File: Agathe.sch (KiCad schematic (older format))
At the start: 153 parts, among them SW1 SW_Push, U1 ATmega32U4-AU, U2 PRTR5V0U2X, Y1 Crystal_GND24_Small

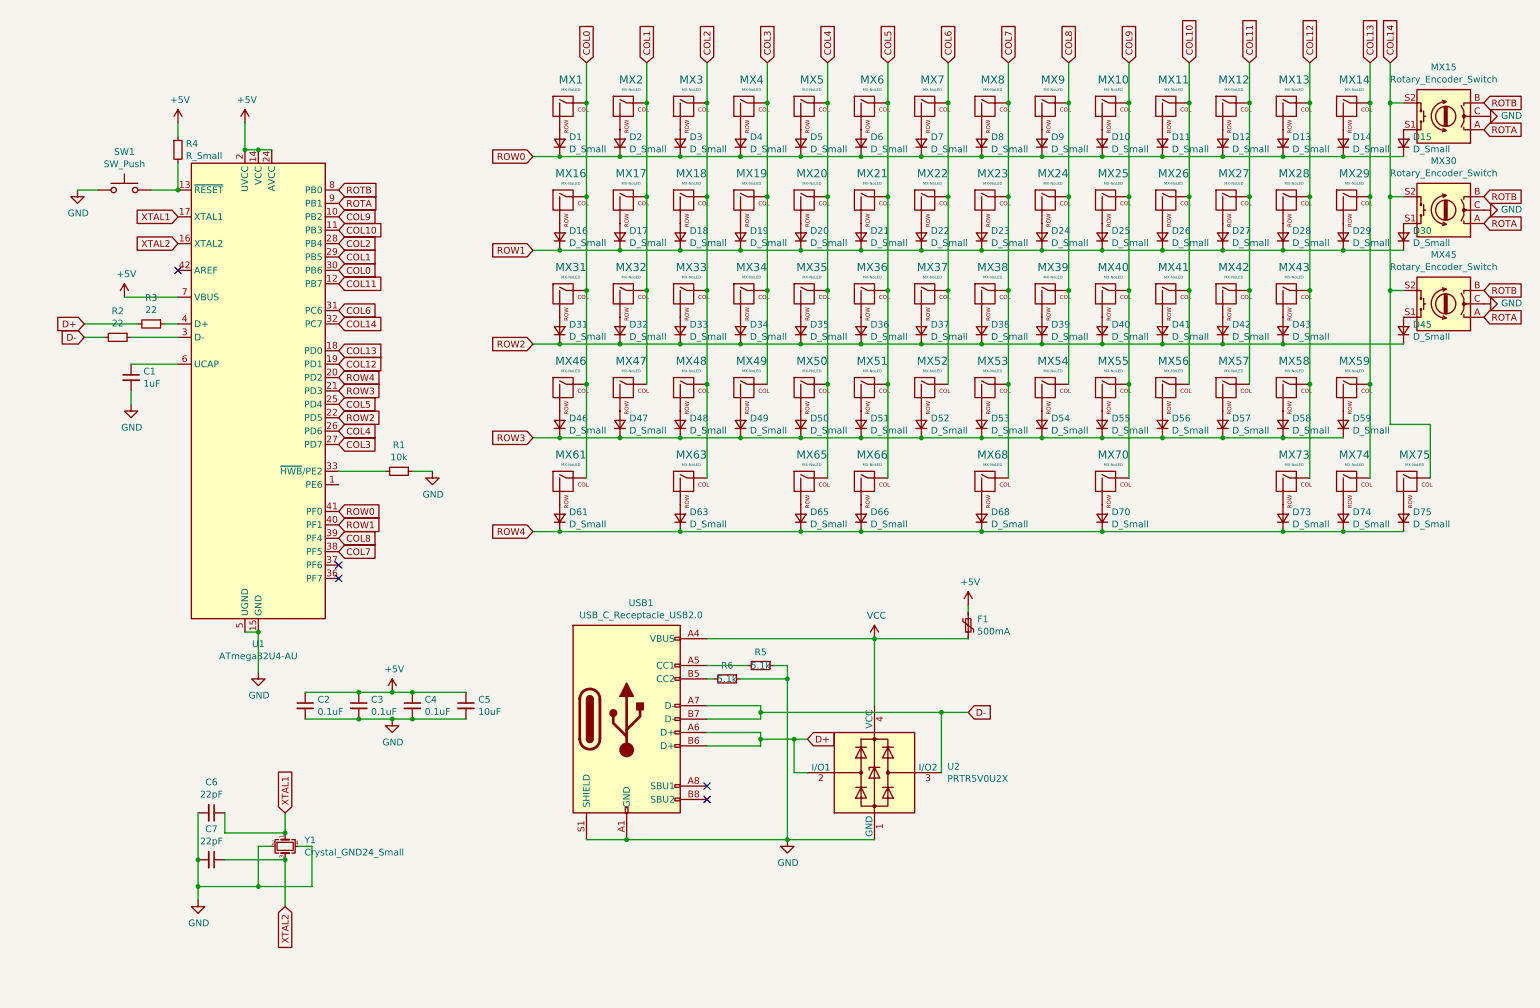
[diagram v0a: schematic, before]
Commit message: Add underglow
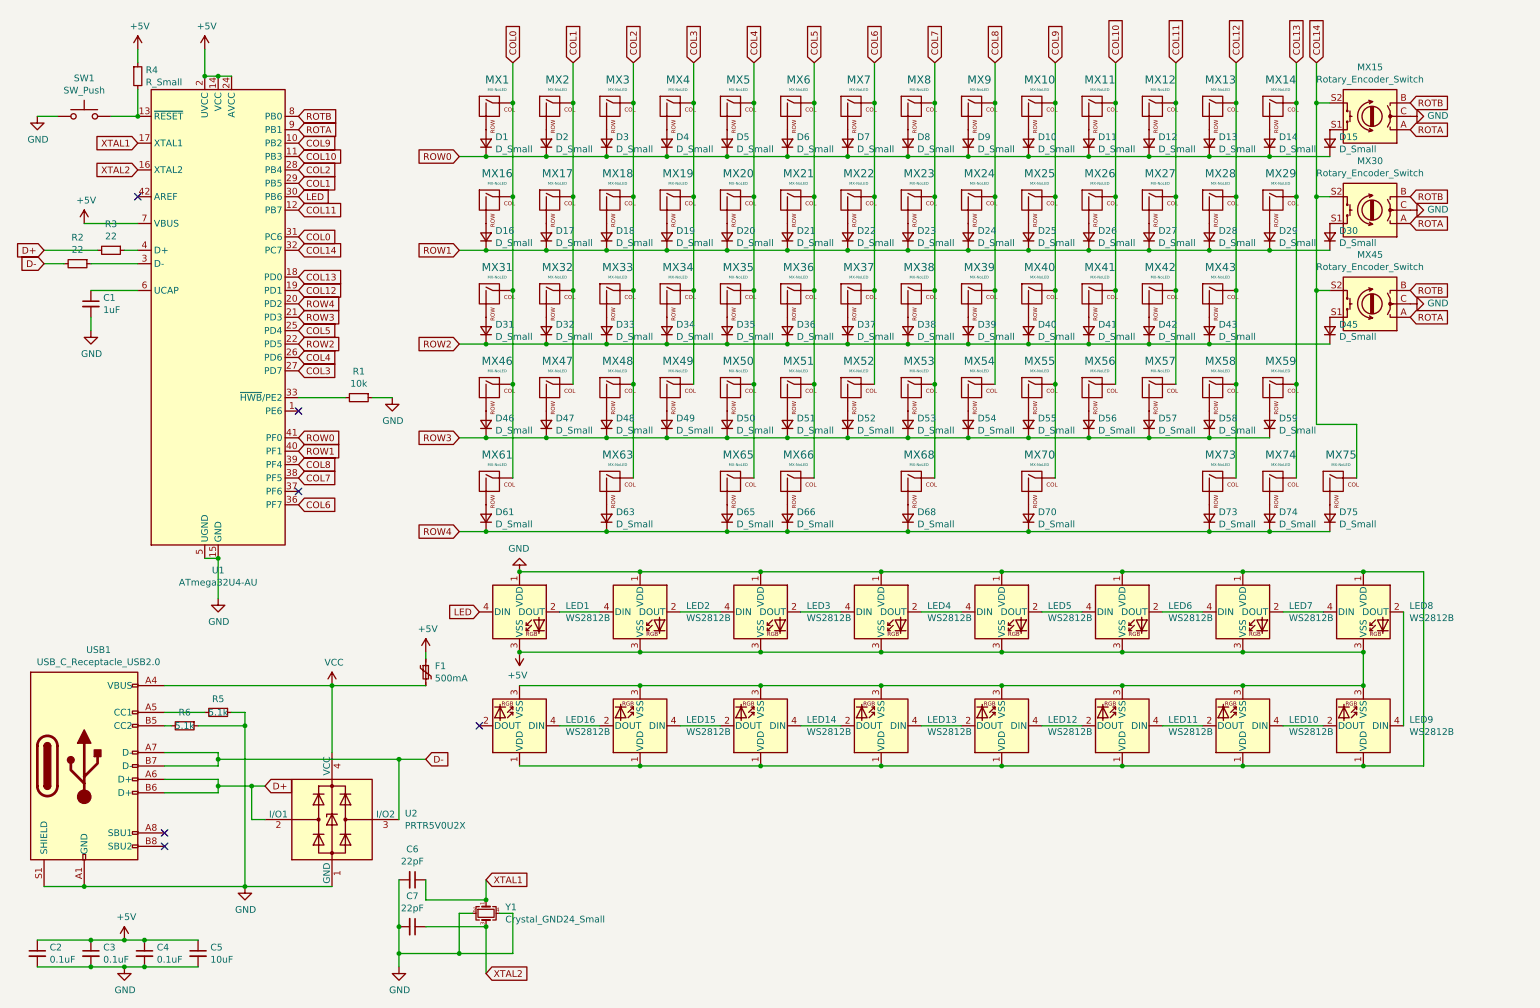
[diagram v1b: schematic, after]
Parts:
- added LED1, LED10, LED11, LED12, LED13, LED14, LED15, LED16, LED2, LED3, LED4, LED5, LED6, LED7, LED8, LED9: WS2812B, LED_SMD:LED_WS2812B_PLCC4_5.0x5.0mm_P3.2mm, symbol LED:WS2812B
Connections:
- net +5V: now also LED1.3 (VSS), LED10.3 (VSS), LED11.3 (VSS), LED12.3 (VSS), LED13.3 (VSS), LED14.3 (VSS), LED15.3 (VSS), LED16.3 (VSS), LED2.3 (VSS), LED3.3 (VSS), LED4.3 (VSS), LED5.3 (VSS), LED6.3 (VSS), LED7.3 (VSS), LED8.3 (VSS), LED9.3 (VSS)
- net COL0: now also U1.31 (PC6); no longer U1.30 (PB6)
- net COL6: now also U1.36 (PF7); no longer U1.31 (PC6)
- net GND: now also LED1.1 (VDD), LED10.1 (VDD), LED11.1 (VDD), LED12.1 (VDD), LED13.1 (VDD), LED14.1 (VDD), LED15.1 (VDD), LED16.1 (VDD), LED2.1 (VDD), LED3.1 (VDD), LED4.1 (VDD), LED5.1 (VDD), LED6.1 (VDD), LED7.1 (VDD), LED8.1 (VDD), LED9.1 (VDD)
- new net: LED2.2 (DOUT), LED3.4 (DIN)
- new net: LED1.2 (DOUT), LED2.4 (DIN)
- new net: LED3.2 (DOUT), LED4.4 (DIN)
- new net: LED4.2 (DOUT), LED5.4 (DIN)
- new net: LED5.2 (DOUT), LED6.4 (DIN)
- new net: LED6.2 (DOUT), LED7.4 (DIN)
- new net: LED7.2 (DOUT), LED8.4 (DIN)
- new net: LED8.2 (DOUT), LED9.4 (DIN)
- new net: LED10.4 (DIN), LED9.2 (DOUT)
- new net: LED10.2 (DOUT), LED11.4 (DIN)
- new net: LED11.2 (DOUT), LED12.4 (DIN)
- new net: LED12.2 (DOUT), LED13.4 (DIN)
- new net: LED13.2 (DOUT), LED14.4 (DIN)
- new net: LED14.2 (DOUT), LED15.4 (DIN)
- new net: LED15.2 (DOUT), LED16.4 (DIN)
- new net LED: LED1.4 (DIN), U1.30 (PB6)
- no-connect marks 5 -> 6
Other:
- moved on the sheet: C1, C2, C3, C4, C5, C6, C7, D1, D10, D11, D12, D13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
